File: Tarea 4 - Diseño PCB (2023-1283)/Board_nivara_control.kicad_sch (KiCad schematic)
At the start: 6 parts, among them U1 ESP32-S3-WROOM-1

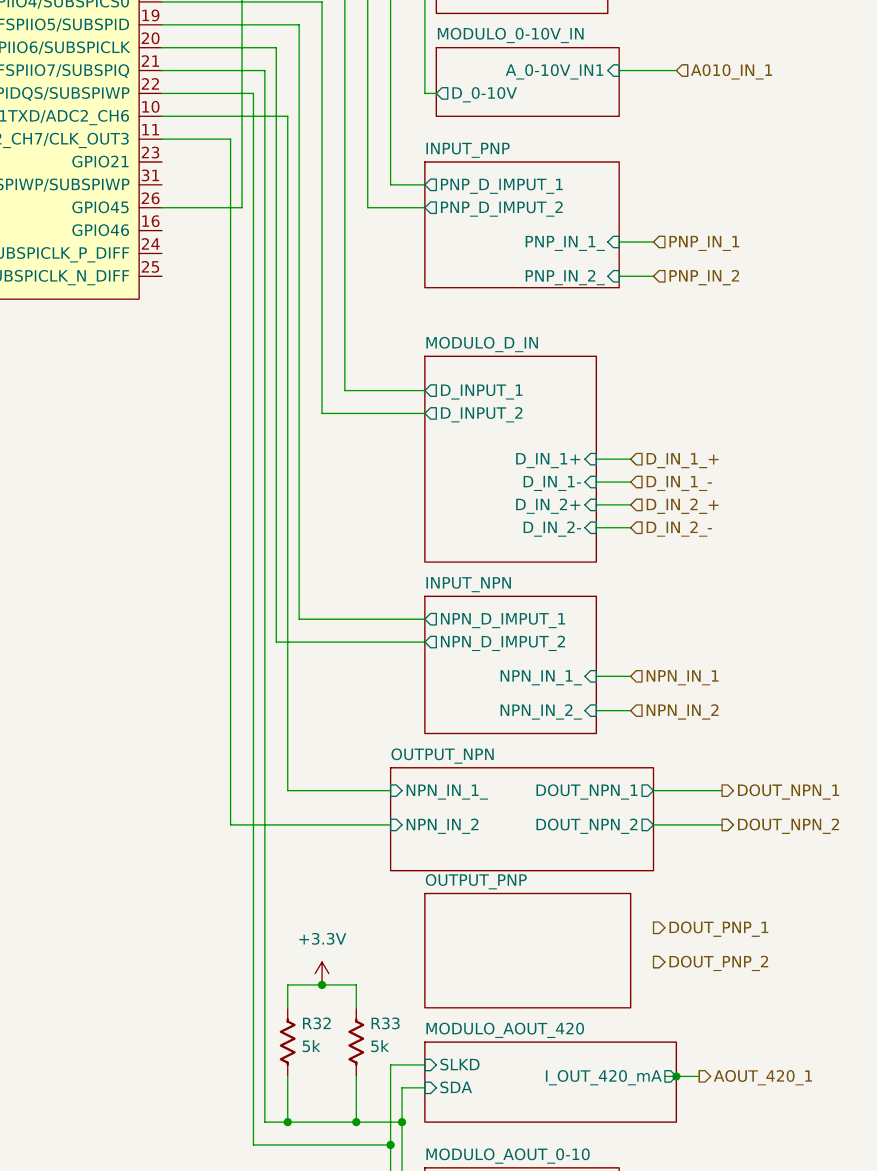
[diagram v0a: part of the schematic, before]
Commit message: Complete
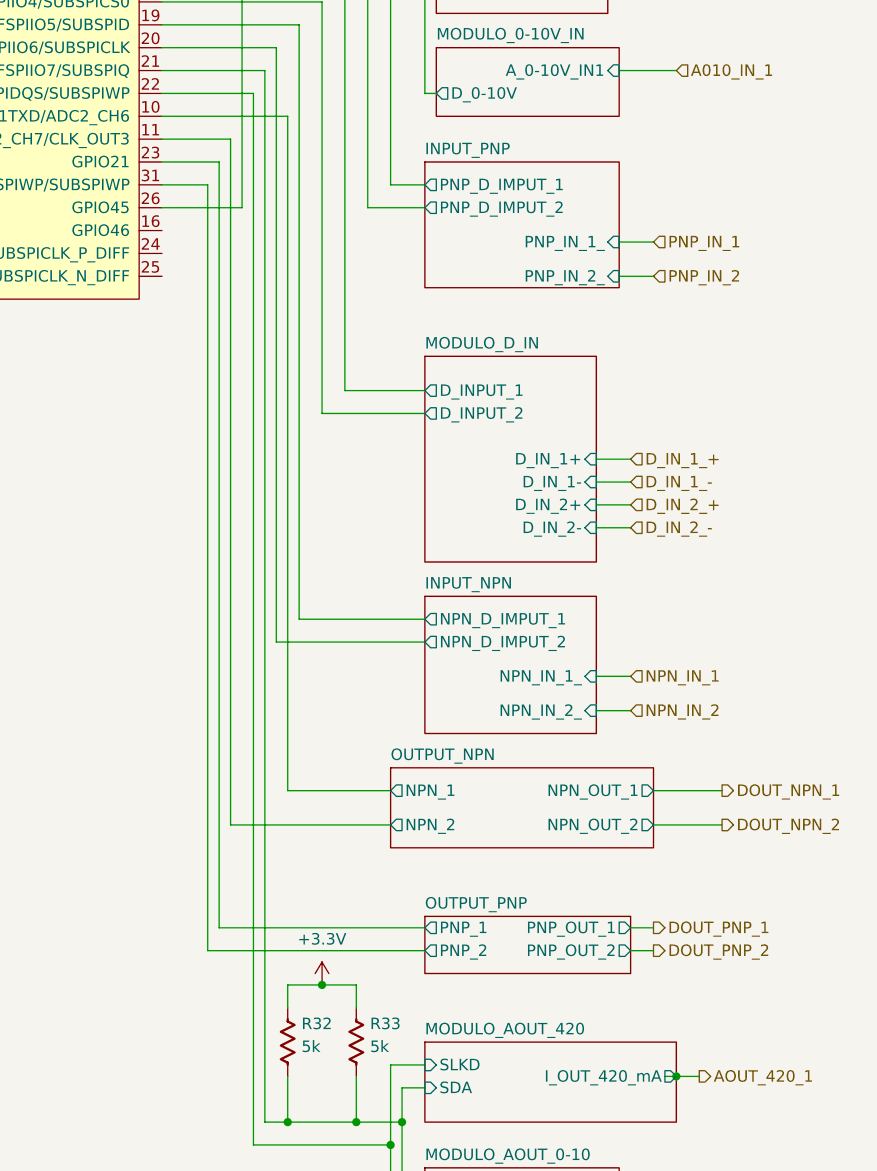
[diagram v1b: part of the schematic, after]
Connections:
- net OUTPUT_PNP/PNP_1: now reaches U1.23 (GPIO21)
- net OUTPUT_PNP/PNP_2: now reaches U1.31 (GPIO38/FSPIWP/SUBSPIWP)
- net OUTPUT_NPN/NPN_IN_1_ renamed OUTPUT_NPN/NPN_1
- net OUTPUT_NPN/NPN_IN_2 renamed OUTPUT_NPN/NPN_2
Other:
- sheet OUTPUT_NPN ports: added NPN_1, NPN_2, NPN_OUT_1, NPN_OUT_2; removed DOUT_NPN_1, DOUT_NPN_2, NPN_IN_1_, NPN_IN_2
- sheet OUTPUT_PNP ports: added PNP_1, PNP_2, PNP_OUT_1, PNP_OUT_2; removed none
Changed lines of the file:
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@@
+	(wire
+		(pts
+			(xy 308.61 184.15) (xy 311.15 184.15)
+		)
+		(stroke
+			(width 0)
+			(type default)
+		)
+	)
 	(wire
 		(pts
@@
 	(wire
 		(pts
+			(xy 262.89 181.61) (xy 285.75 181.61)
+		)
+		(stroke
+			(width 0)
+			(type default)
+		)
+	)
+	(wire
+		(pts
 			(xy 270.51 166.37) (xy 270.51 91.44)
 		)
@@
 	(wire
 		(pts
+			(xy 261.62 99.06) (xy 256.54 99.06)
+		)
+		(stroke
+			(width 0)
+			(type default)
+		)
+	)
+	(wire
+		(pts
 			(xy 259.08 44.45) (xy 259.08 55.88)
 		)
@@
 	(wire
 		(pts
+			(xy 308.61 181.61) (xy 311.15 181.61)
+		)
+		(stroke
+			(width 0)
+			(type default)
+		)
+	)
+	(wire
+		(pts
 			(xy 295.91 29.21) (xy 297.18 29.21)
 		)
@@
 	(wire
 		(pts
+			(xy 256.54 96.52) (xy 262.89 96.52)
+		)
+		(stroke
+			(width 0)
+			(type default)
+		)
+	)
+	(wire
+		(pts
 			(xy 259.08 55.88) (xy 256.54 55.88)
 		)
@@
 	(wire
 		(pts
+			(xy 262.89 96.52) (xy 262.89 181.61)
+		)
+		(stroke
+			(width 0)
+			(type default)
+		)
+	)
+	(wire
+		(pts
 			(xy 306.07 68.58) (xy 311.15 68.58)
 		)
@@
 		(pts
 			(xy 285.75 101.6) (xy 279.4 101.6)
+		)
+		(stroke
+			(width 0)
+			(type default)
+		)
+	)
+	(wire
+		(pts
+			(xy 285.75 184.15) (xy 261.62 184.15)
+		)
+		(stroke
+			(width 0)
+			(type default)
+		)
+	)
+	(wire
+		(pts
+			(xy 261.62 184.15) (xy 261.62 99.06)
 		)
 		(stroke
@@
 	(hierarchical_label "DOUT_PNP_2"
 		(shape output)
-		(at 311.15 185.42 0)
+		(at 311.15 184.15 0)
 		(effects
 			(font
@@
 	)
 	(sheet
-		(at 285.75 177.8)
-		(size 22.86 12.7)
+		(at 285.75 180.34)
+		(size 22.86 6.35)
 		(exclude_from_sim no)
 		(in_bom yes)
@@
 		)
 		(property "Sheetname" "OUTPUT_PNP"
-			(at 285.75 177.0884 0)
+			(at 285.75 179.6284 0)
 			(effects
 				(font
@@
 		)
 		(property "Sheetfile" "OUTPUT_PNP.kicad_sch"
-			(at 285.75 191.0846 0)
+			(at 285.75 187.2746 0)
 			(effects
 				(font
@@
 				(justify left top)
 				(hide yes)
+			)
+		)
+		(pin "PNP_1" output
+			(at 285.75 181.61 180)
+			(effects
+				(font
+					(size 1.27 1.27)
+				)
+				(justify left)
+			)
+		)
+		(pin "PNP_2" output
+			(at 285.75 184.15 180)
+			(effects
+				(font
+					(size 1.27 1.27)
+				)
+				(justify left)
+			)
+		)
+		(pin "PNP_OUT_1" output
+			(at 308.61 181.61 0)
+			(effects
+				(font
+					(size 1.27 1.27)
+				)
+				(justify right)
+			)
+		)
+		(pin "PNP_OUT_2" output
+			(at 308.61 184.15 0)
+			(effects
+				(font
+					(size 1.27 1.27)
+				)
+				(justify right)
 			)
 		)
@@
 	(sheet
 		(at 281.94 163.83)
-		(size 29.21 11.43)
+		(size 29.21 8.89)
 		(exclude_from_sim no)
 		(in_bom yes)
@@
 		)
 		(property "Sheetfile" "OUTPUT_NPN.kicad_sch"
-			(at 281.94 175.8446 0)
+			(at 281.94 173.3046 0)
 			(effects
 				(font
@@
 			)
 		)
-		(pin "DOUT_NPN_1" output
+		(pin "NPN_1" output
+			(at 281.94 166.37 180)
+			(effects
+				(font
+					(size 1.27 1.27)
+				)
+				(justify left)
+			)
+		)
+		(pin "NPN_2" output
+			(at 281.94 170.18 180)
+			(effects
+				(font
+					(size 1.27 1.27)
+				)
+				(justify left)
+			)
+		)
+		(pin "NPN_OUT_1" output
 			(at 311.15 166.37 0)
 			(effects
@@
 			)
 		)
-		(pin "NPN_IN_1_" input
-			(at 281.94 166.37 180)
-			(effects
-				(font
-					(size 1.27 1.27)
-				)
-				(justify left)
-			)
-		)
-		(pin "NPN_IN_2" input
-			(at 281.94 170.18 180)
-			(effects
-				(font
-					(size 1.27 1.27)
-				)
-				(justify left)
-			)
-		)
-		(pin "DOUT_NPN_2" output
+		(pin "NPN_OUT_2" output
 			(at 311.15 170.18 0)
 			(effects
